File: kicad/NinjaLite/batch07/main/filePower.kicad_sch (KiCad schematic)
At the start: 28 parts, among them J1 ALI_USB, J2 Barrel_Jack_Switch, Q1 Q_NMOS_GSD, U11 IP2721, U14 TCR3DF33,LM(CT, U3 BD433M5FP-CE2, U6 BA178M05FP-E2, U7 BD433M5FP-CE2

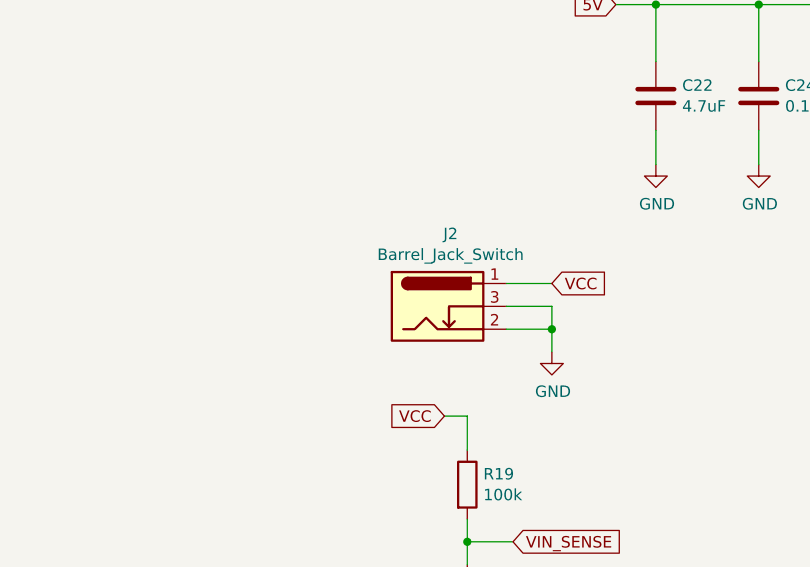
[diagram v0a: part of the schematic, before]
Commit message: sync
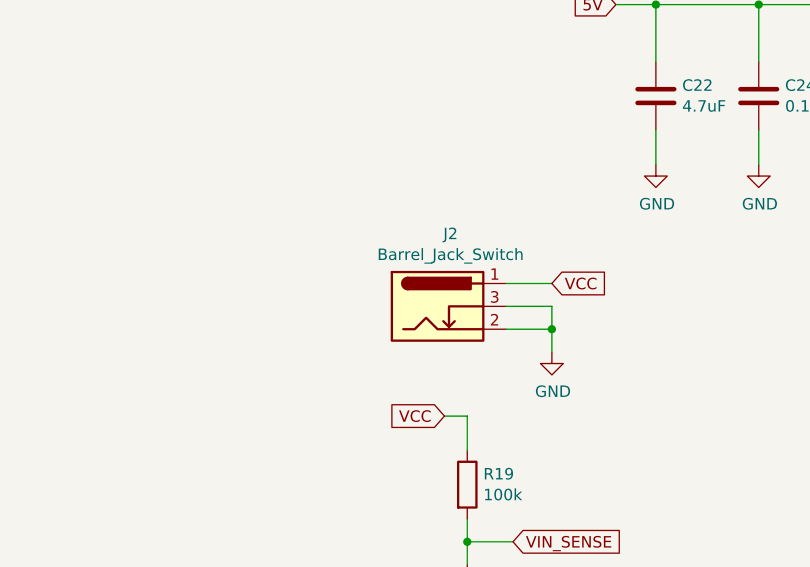
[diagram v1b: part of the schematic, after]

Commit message: wiring batch7
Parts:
- C23: footprint Ninja-qPCR:35TZV100M6.3X8 -> Ninja:35TZV100M6.3X8
- J1: footprint Ninja-qPCR:ALI_USB -> Ninja:ALI_USB
- Q1: footprint Ninja-qPCR:SOT95P240X112-3N -> Ninja:SOT95P240X112-3N
- U3, U6: footprint Ninja-qPCR:REG_TO252-3 -> Ninja:REG_TO252-3
- U7: footprint Ninja-qPCR:REG_TO252-3-INV -> Ninja:REG_TO252-3-INV
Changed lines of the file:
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@@
       (effects (font (size 1.27 1.27)))
     )
-    (property "Footprint" "Ninja-qPCR:REG_TO252-3" (at 227.965 70.485 0)
+    (property "Footprint" "Ninja:REG_TO252-3" (at 227.965 70.485 0)
       (effects (font (size 1.27 1.27)) hide)
     )
@@
       (effects (font (size 1.27 1.27)))
     )
-    (property "Footprint" "Ninja-qPCR:ALI_USB" (at 38.1 58.42 0)
+    (property "Footprint" "Ninja:ALI_USB" (at 38.1 58.42 0)
       (effects (font (size 1.27 1.27)) hide)
     )
@@
       (effects (font (size 1.27 1.27)))
     )
-    (property "Footprint" "Ninja-qPCR:REG_TO252-3" (at 227.965 41.275 0)
+    (property "Footprint" "Ninja:REG_TO252-3" (at 227.965 41.275 0)
       (effects (font (size 1.27 1.27)) hide)
     )
@@
       (effects (font (size 1.27 1.27)))
     )
-    (property "Footprint" "Ninja-qPCR:SOT95P240X112-3N" (at 60.96 41.91 0)
+    (property "Footprint" "Ninja:SOT95P240X112-3N" (at 60.96 41.91 0)
       (effects (font (size 1.27 1.27)) hide)
     )
@@
       (effects (font (size 1.27 1.27)) (justify left))
     )
-    (property "Footprint" "Ninja-qPCR:35TZV100M6.3X8" (at 181.9402 57.785 0)
+    (property "Footprint" "Ninja:35TZV100M6.3X8" (at 181.9402 57.785 0)
       (effects (font (size 1.27 1.27)) hide)
     )
@@
       (effects (font (size 1.27 1.27)))
     )
-    (property "Footprint" "Ninja-qPCR:REG_TO252-3-INV" (at 250.444 21.59 0)
-      (effects (font (size 1.27 1.27)) hide)
-    )
+    (property "Footprint" "Ninja:REG_TO252-3-INV" (at 250.444 21.59 0)
+      (effects (font (size 1.27 1.27)) hide)
+    )
